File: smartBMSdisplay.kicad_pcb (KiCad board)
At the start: 2 copper layers, 95.9 x 45.1 mm, 11 parts, among them J1 Conn_01x04_Male, J2 Conn_01x05_Male, Q1 BC547

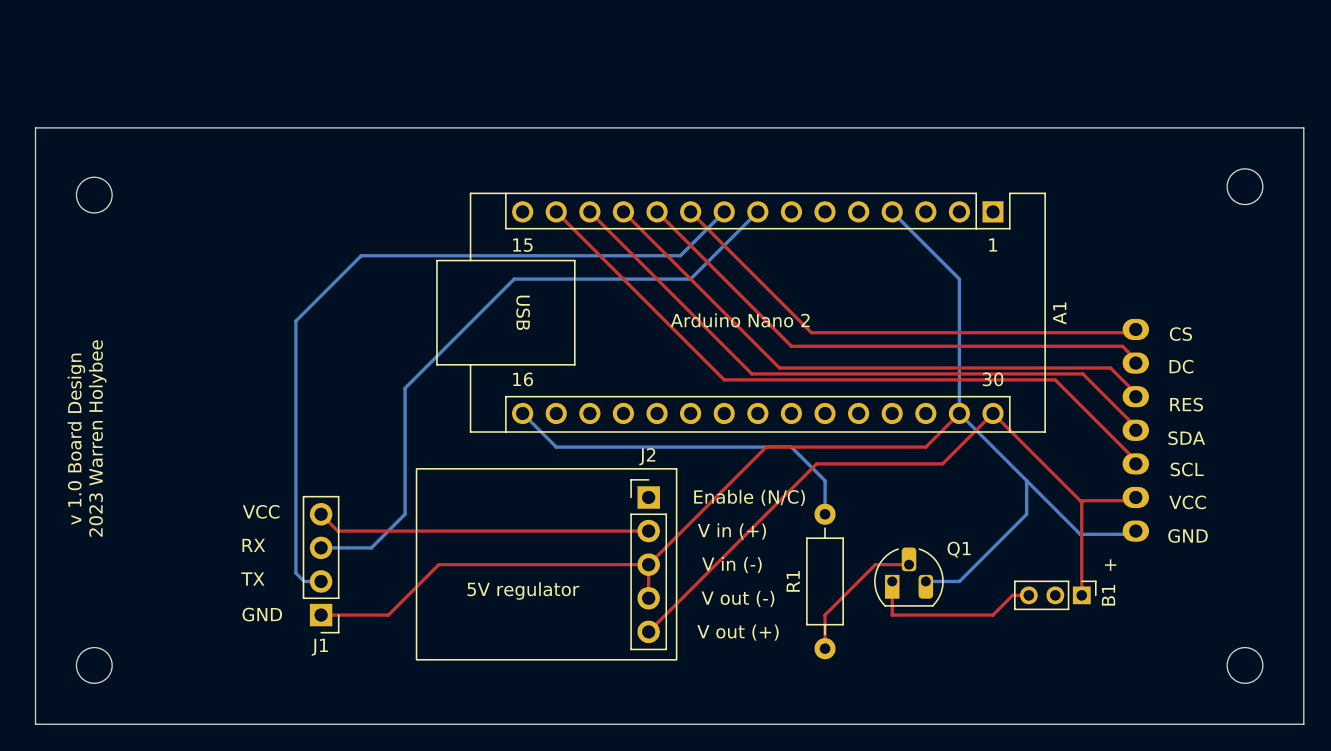
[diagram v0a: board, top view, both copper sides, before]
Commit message: First working bluetooth version
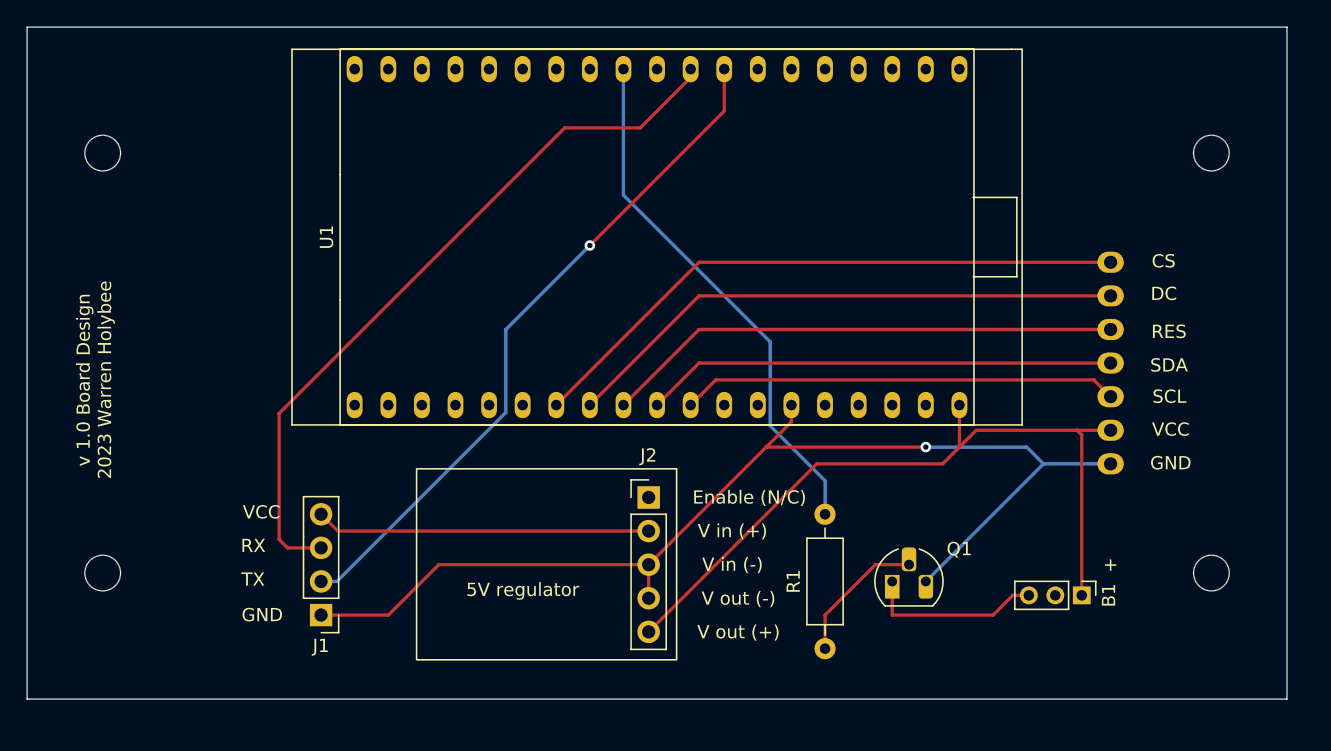
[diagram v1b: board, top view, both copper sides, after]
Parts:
- removed A1: Arduino_Nano_v2.x, Module:Arduino_Nano
- added U1: esp32_WROOM, ESP32-smartBMSdisplay:ESP32_Devkit_38Pins, F.Cu at (149.9, 73.0)
- moved H4 7.43 mm to (191.8, 98.4)
- moved H2 7.01 mm to (108.0, 98.4)
- moved Brd1 5.43 mm to (171.4, 82.5)
- moved H3 3.59 mm to (191.8, 66.7)
- moved H1 3.24 mm to (108.0, 66.7)
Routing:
- net GND: track 104.3 -> 84.6 mm, vias 0 -> 1
- net Net-(Brd1-Pad3): track 52.3 -> 33.1 mm
- net Net-(Brd1-Pad4): track 48.7 -> 35.6 mm
- net Net-(R1-Pad2): track 27.5 -> 40.0 mm
- net Net-(Brd1-Pad7): track 37.9 -> 46.4 mm
- net Net-(J1-Pad3): track 49.1 -> 55.2 mm
- net Net-(Brd1-Pad5): track 45.1 -> 39.2 mm
- net Net-(J1-Pad2): track 57.0 -> 52.1 mm, vias 0 -> 1
- net Net-(B1-Pad1): track 54.1 -> 57.0 mm
- net Net-(Brd1-Pad6): track 41.5 -> 42.8 mm
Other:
- board size 95.9 x 45.1 mm -> 95.3 x 50.8 mm
- board text removed: "1"
- board text removed: "15"
- board text removed: "16"
- board text removed: "30"
- board text removed: "Arduino Nano 2"
- board text removed: "SSD 1309 128x64 2.52{dblquote} SPI Interface"
